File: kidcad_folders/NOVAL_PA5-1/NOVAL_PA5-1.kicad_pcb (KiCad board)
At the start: 2 copper layers, 75.5 x 45.5 mm, 10 parts, among them J1 Conn_01x01_Pin, J2 Conn_01x01_Pin, M2 Motor_DC, M3 Motor_DC, M4 Motor_Servo, M5 Motor_DC, M7 Motor_Servo_AirTronics, M8 Motor_Servo_AirTronics, U1 L293D, U2 L293D

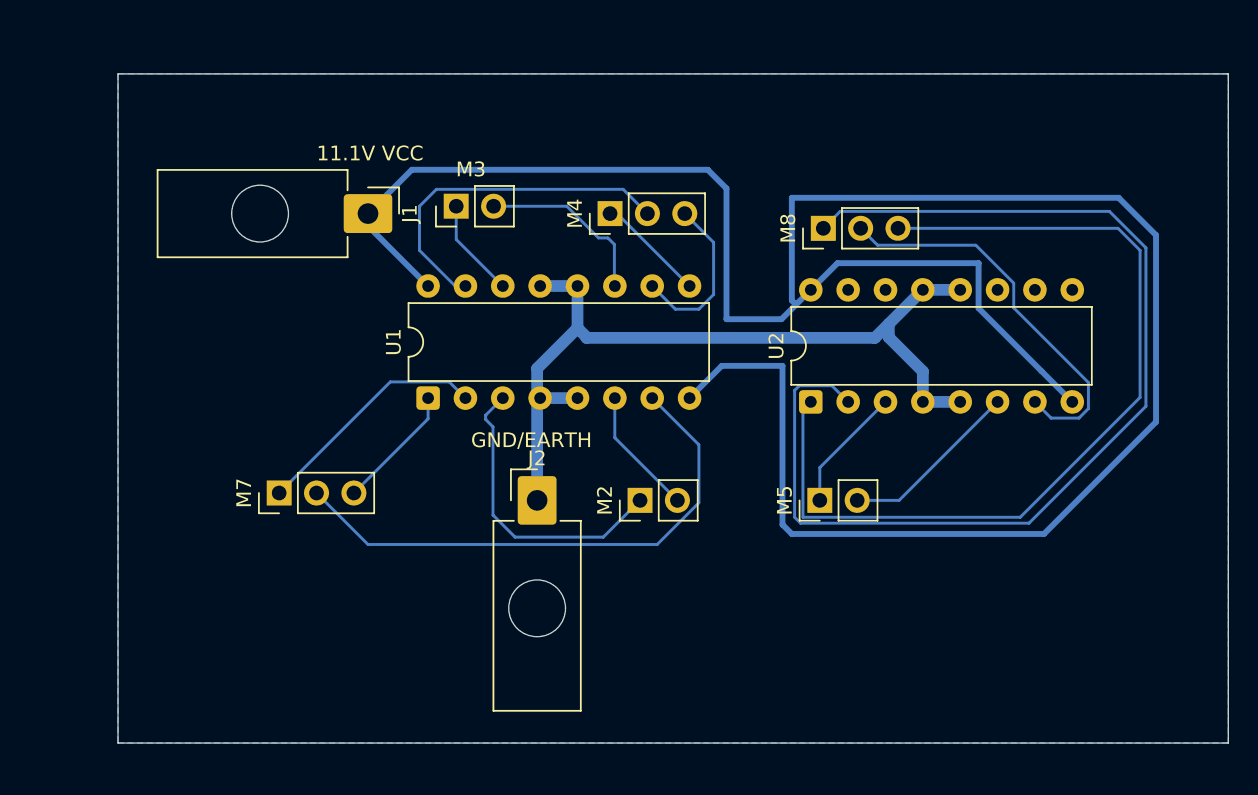
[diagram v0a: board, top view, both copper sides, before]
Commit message: PA5-1
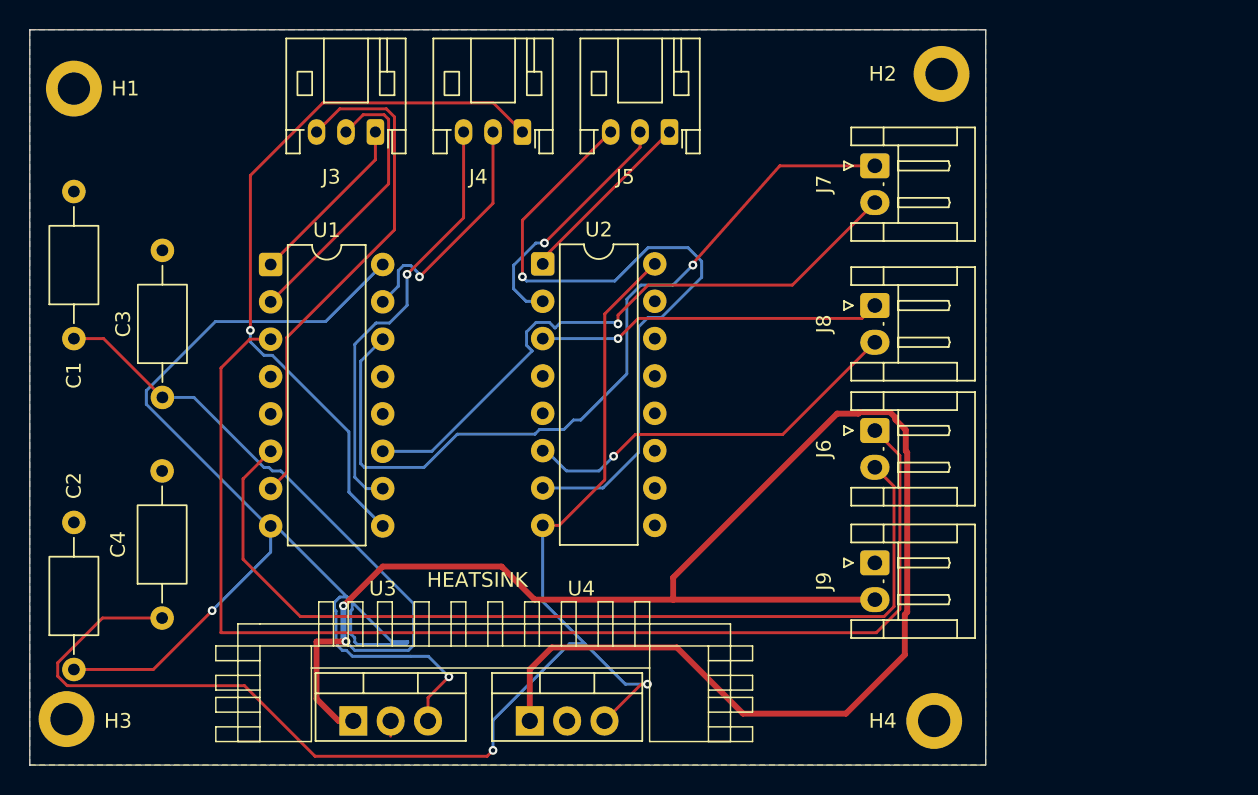
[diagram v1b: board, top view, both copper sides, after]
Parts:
- removed J1, J2: Conn_01x01_Pin, Connector_TE-Connectivity:TE_MATE-N-LOK_1-794374-x_1x01_P4.14mm_Horizontal
- removed M2, M3, M5: Motor_DC, Connector_PinHeader_2.54mm:PinHeader_1x02_P2.54mm_Vertical
- removed M4: Motor_Servo, Connector_PinHeader_2.54mm:PinHeader_1x03_P2.54mm_Vertical
- removed M7, M8: Motor_Servo_AirTronics, Connector_PinHeader_2.54mm:PinHeader_1x03_P2.54mm_Vertical
- added C1: C_US, Capacitor_THT:C_Axial_L5.1mm_D3.1mm_P10.00mm_Horizontal, F.Cu at (98.5, 108.0)
- added C2: C_US, Capacitor_THT:C_Axial_L5.1mm_D3.1mm_P10.00mm_Horizontal, F.Cu at (98.5, 130.5)
- added C3: C_US, Capacitor_THT:C_Axial_L5.1mm_D3.1mm_P10.00mm_Horizontal, F.Cu at (104.5, 112.0)
- added C4: C_US, Capacitor_THT:C_Axial_L5.1mm_D3.1mm_P10.00mm_Horizontal, F.Cu at (104.5, 127.0)
- added H1: MountingHole_Pad, MountingHole:MountingHole_2.2mm_M2_DIN965_Pad, F.Cu at (98.5, 91.0)
- added H2: MountingHole_Pad, MountingHole:MountingHole_2.2mm_M2_DIN965_Pad, F.Cu at (157.5, 90.0)
- added H3: MountingHole_Pad, MountingHole:MountingHole_2.2mm_M2_DIN965_Pad, F.Cu at (98.0, 133.9)
- added H4: MountingHole_Pad, MountingHole:MountingHole_2.2mm_M2_DIN965_Pad, F.Cu at (157.0, 134.0)
- added J3: Conn_01x03_Pin, Connector_JST:JST_PH_S3B-PH-K_1x03_P2.00mm_Horizontal, F.Cu at (119.0, 94.0)
- added J4: Conn_01x03_Pin, Connector_JST:JST_PH_S3B-PH-K_1x03_P2.00mm_Horizontal, F.Cu at (129.0, 94.0)
- added J5: Conn_01x03_Pin, Connector_JST:JST_PH_S3B-PH-K_1x03_P2.00mm_Horizontal, F.Cu at (139.0, 94.0)
- added J6: Conn_01x02_Pin, Connector_JST:JST_EH_S2B-EH_1x02_P2.50mm_Horizontal, F.Cu at (153.0, 114.2)
- added J7: Conn_01x02_Pin, Connector_JST:JST_EH_S2B-EH_1x02_P2.50mm_Horizontal, F.Cu at (153.0, 96.2)
- added J8: Conn_01x02_Pin, Connector_JST:JST_EH_S2B-EH_1x02_P2.50mm_Horizontal, F.Cu at (153.0, 105.8)
- added J9: Conn_01x02_Pin, Connector_JST:JST_EH_S2B-EH_1x02_P2.50mm_Horizontal, F.Cu at (153.0, 123.2)
- added REF**: HEATSINKUSV, Custom_stuff:HEATSINKUSV, F.Cu at (177.7, 146.9)
- added U3: L7805, Package_TO_SOT_THT:TO-220-3_Vertical, F.Cu at (117.5, 134.0)
- added U4: L7805, Package_TO_SOT_THT:TO-220-3_Vertical, F.Cu at (129.5, 134.0)
- moved U2 20.5 mm to (130.4, 102.9), turned to 0 degrees
- moved U1 14.0 mm to (111.9, 103.0), turned to 0 degrees
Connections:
- U1 pad 16: 11.1V -> Net-(U1-VCC1)
- U1 pad 8: 11.1V -> Net-(U1-VCC1)
- U2 pad 16: 11.1V -> Net-(U2-VCC1)
- U2 pad 8: 11.1V -> Net-(U2-VCC1)
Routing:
- net Net-(U2-VCC1): track 0.00 -> 91.2 mm, vias 0 -> 2
- net Net-(U1-VCC1): track 0.00 -> 87.0 mm, vias 0 -> 2
- net /MOTOR1A: track 20.3 -> 81.9 mm
- net /FDIRECTION3: track 74.4 -> 16.9 mm, vias 0 -> 1
- net GND: track 57.6 -> 1.04 mm
- net /MOTOR1B: track 8.72 -> 64.3 mm
- net /PWM3: track 61.4 -> 12.5 mm
- net /PWM2: track 7.45 -> 49.3 mm, vias 0 -> 1
- net /MOTOR2A: track 6.74 -> 47.1 mm, vias 0 -> 1
- net /MOTOR2B: track 9.29 -> 42.5 mm, vias 0 -> 1
- net /BDIRECTION3: track 27.0 -> 48.8 mm, vias 0 -> 1
- net /BDIRECTION2: track 11.6 -> 29.3 mm, vias 0 -> 1
- net /MOTOR3A: track 8.54 -> 23.5 mm, vias 0 -> 1
- net /MOTOR3B: track 12.3 -> 26.8 mm, vias 0 -> 1
- net /FDIRECTION2: track 23.8 -> 16.5 mm, vias 0 -> 1
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- added copper zone on F.Cu, net GND
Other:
- board size 75.5 x 45.5 mm -> 65 x 50 mm
- board text added: "HEATSINK"
- board text removed: "11.1V VCC"
- board text removed: "CpE 2303L-2026 Rev 1.2"
- board text removed: "GND/EARTH"
